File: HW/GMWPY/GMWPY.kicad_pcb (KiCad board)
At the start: 4 copper layers, 13 parts, among them U1 USEQGCDACH4100, U2 TSV991ILT, U3 TSV991ILT

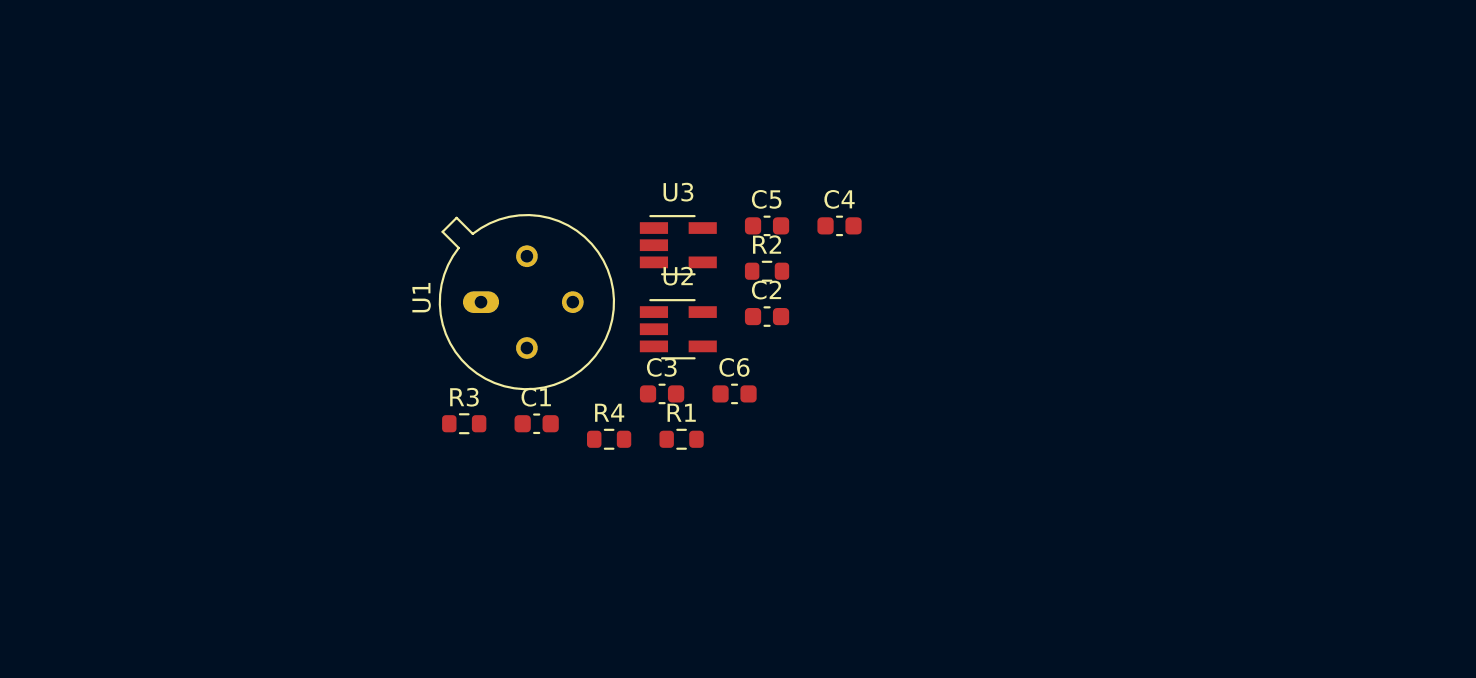
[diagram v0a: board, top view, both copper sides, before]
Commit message: r
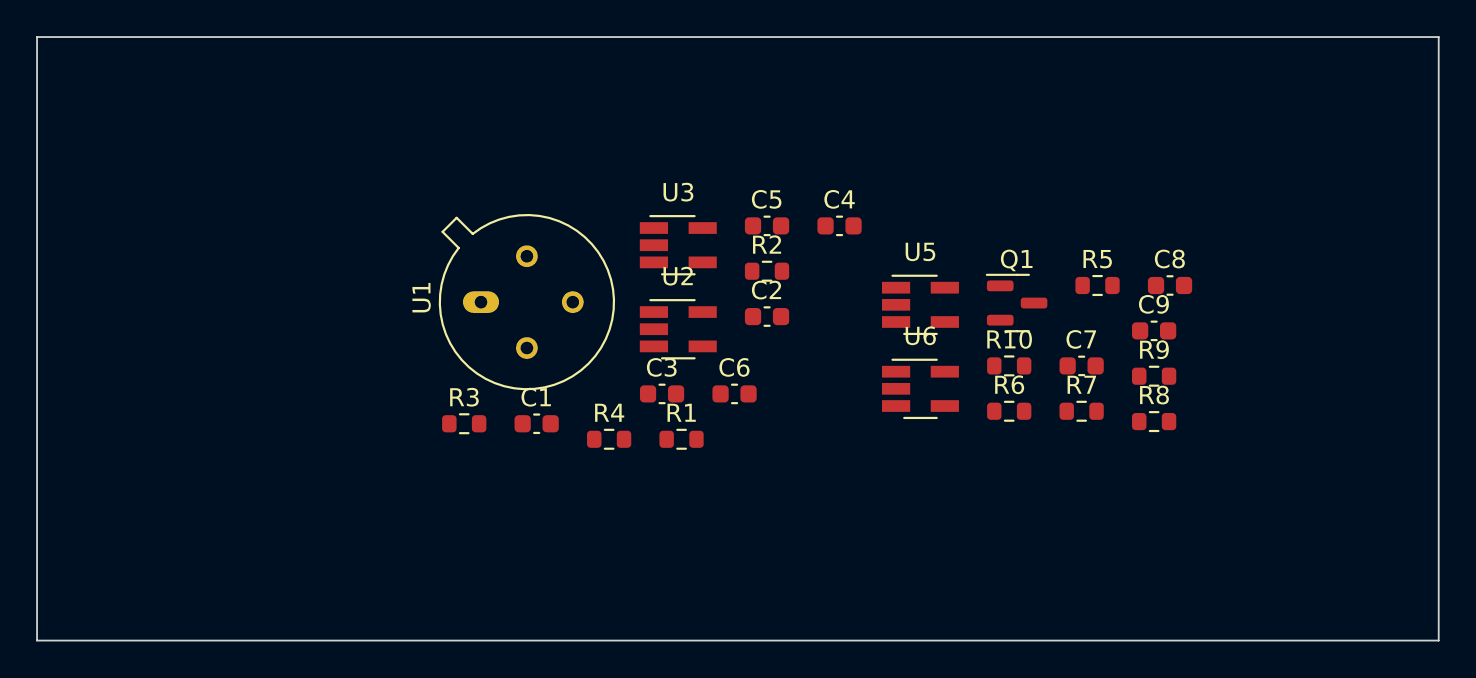
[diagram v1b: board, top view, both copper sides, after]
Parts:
- added C7: 100n, Capacitor_SMD:C_0603_1608Metric, F.Cu at (142.0, 101.8)
- added C8: 100n, Capacitor_SMD:C_0603_1608Metric, F.Cu at (146.9, 97.3)
- added C9: 100n, Capacitor_SMD:C_0603_1608Metric, F.Cu at (146.0, 99.9)
- added Q1: Q_PJFET_DSG, Package_TO_SOT_SMD:SOT-23, F.Cu at (138.5, 98.3)
- added R10: 10k, Resistor_SMD:R_0603_1608Metric, F.Cu at (138.0, 101.8)
- added R5: 1Meg, Resistor_SMD:R_0603_1608Metric, F.Cu at (142.9, 97.3)
- added R6: 10k, Resistor_SMD:R_0603_1608Metric, F.Cu at (138.0, 104.3)
- added R7: 10k, Resistor_SMD:R_0603_1608Metric, F.Cu at (142.0, 104.3)
- added R8: 10, Resistor_SMD:R_0603_1608Metric, F.Cu at (146.0, 104.9)
- added R9: 10, Resistor_SMD:R_0603_1608Metric, F.Cu at (146.0, 102.4)
- added U5: TSV991ILT, Package_TO_SOT_SMD:SOT-23-5_HandSoldering, F.Cu at (133.1, 98.4)
- added U6: TSV991ILT, Package_TO_SOT_SMD:SOT-23-5_HandSoldering, F.Cu at (133.1, 103.1)
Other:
- board outline added: 77.6 x 33.4 mm
